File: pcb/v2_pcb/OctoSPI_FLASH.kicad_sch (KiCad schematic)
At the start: 7 parts, among them U5 MX25U51279GXDR00

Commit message: small
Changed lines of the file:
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@@
-	(wire
-		(pts
-			(xy 127 76.2) (xy 123.19 76.2)
-		)
-		(stroke
-			(width 0)
-			(type default)
-		)
-	)
 	(wire
 		(pts
@@
 	(wire
 		(pts
-			(xy 123.19 76.2) (xy 69.85 76.2)
+			(xy 69.85 76.2) (xy 127 76.2)
 		)
 		(stroke
@@
 		)
 	)
-	(embedded_fonts no)
 )

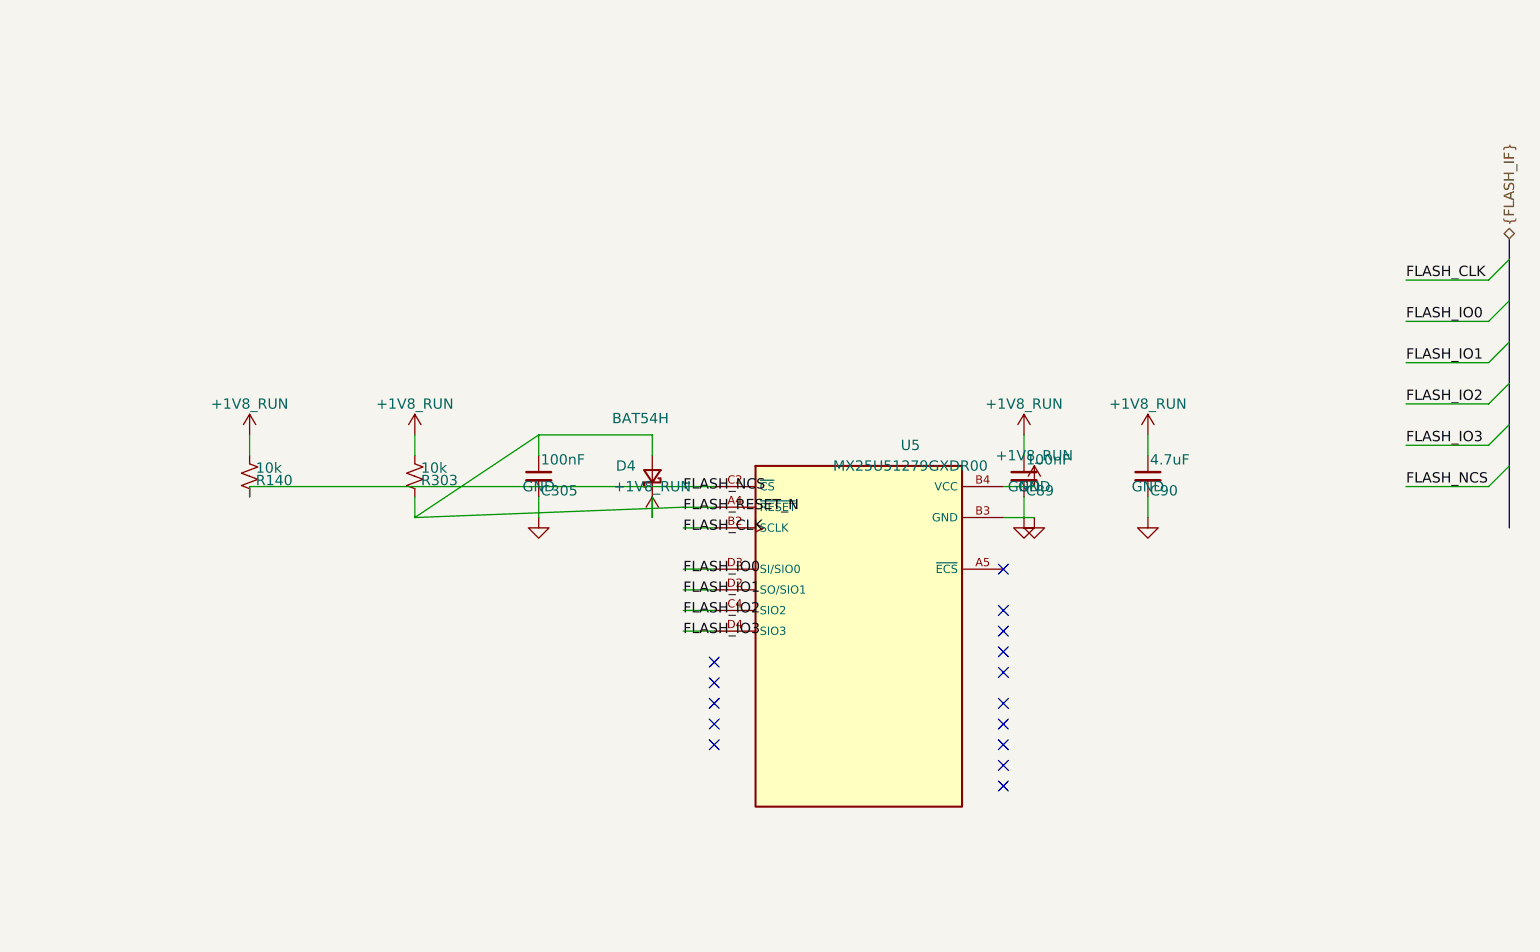
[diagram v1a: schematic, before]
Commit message: minor fixes
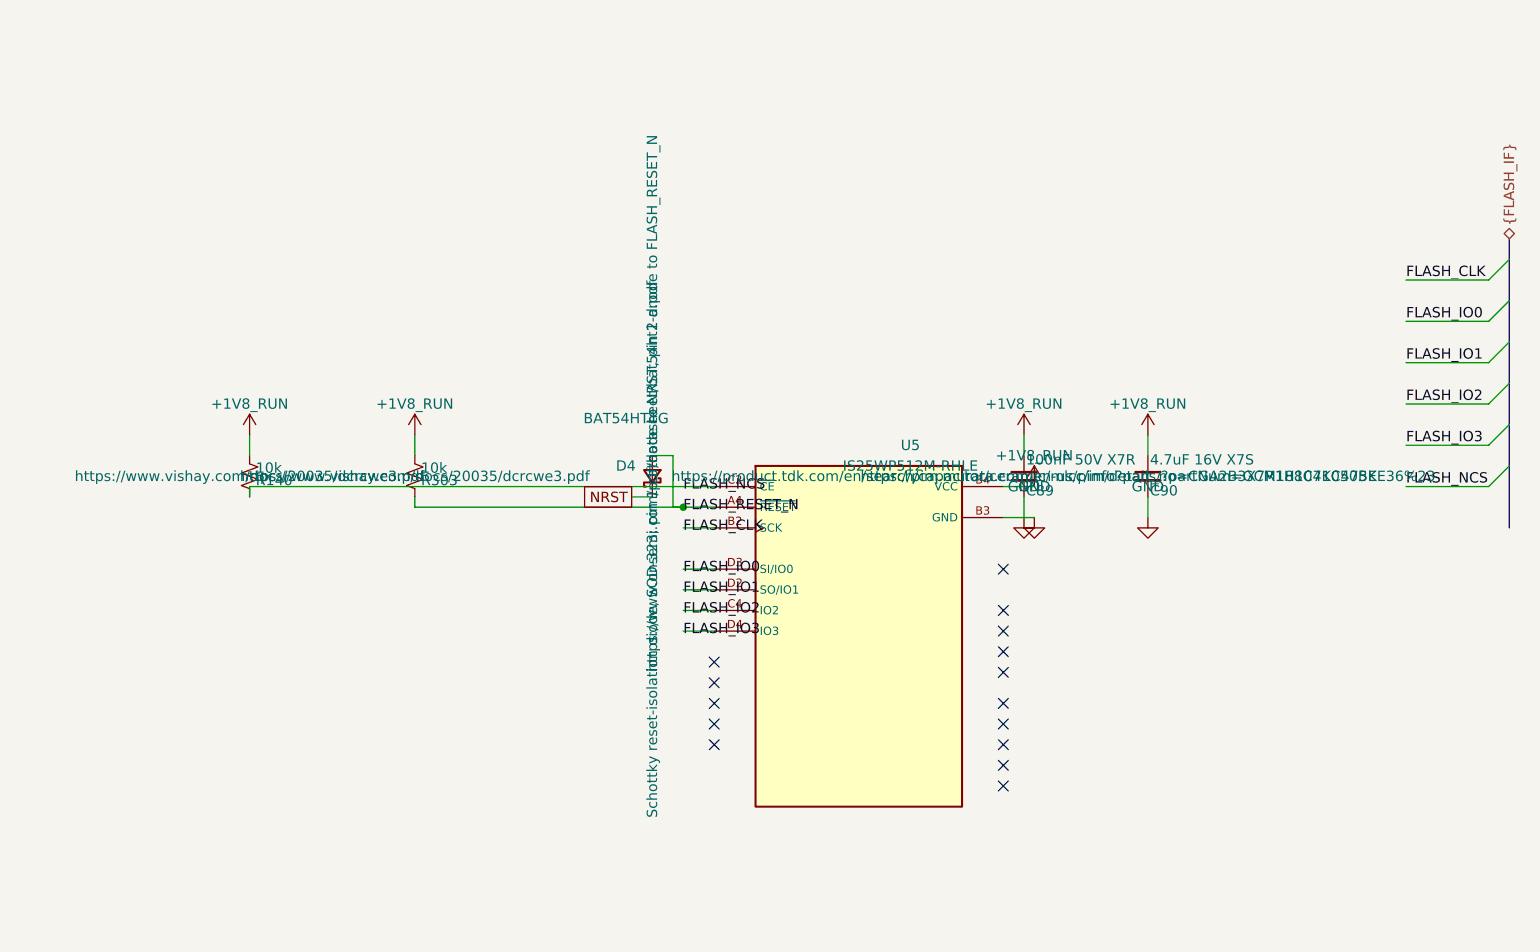
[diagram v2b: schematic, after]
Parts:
- removed C305: 100nF, Capacitor_SMD:C_0402_1005Metric, symbol Device:C_Small
- C89: value 100nF -> 100nF 50V X7R; Dielectric (none) -> X7R; MPN (none) -> CGA2B3X7R1H104K050BE; Manufacturer (none) -> TDK; Qualification (none) -> AEC-Q200; Termination (none) -> Soft termination; Tolerance (none) -> ±10%; Voltage (none) -> 50 VDC
- C90: value 4.7uF -> 4.7uF 16V X7S; Dielectric (none) -> X7S; MPN (none) -> GCM188C71C475KE36D; Manufacturer (none) -> Murata; Qualification (none) -> AEC-Q200 powertrain/safety; Tolerance (none) -> ±10%; Voltage (none) -> 16 VDC
- D4: value BAT54H -> BAT54HT1G; MPN BAT54H,115 -> BAT54HT1G; Manufacturer Nexperia -> onsemi
- R140: MPN (none) -> CRCW040210K0FKED; Manufacturer (none) -> Vishay; Power (none) -> 0.063 W; TCR (none) -> ±100 ppm/K; Tolerance (none) -> ±1%
- R303: MPN (none) -> CRCW040210K0FKED; Manufacturer (none) -> Vishay; Power (none) -> 0.063 W; Qualification (none) -> AEC-Q200; TCR (none) -> ±100 ppm/K; Tolerance (none) -> ±1%
- U5: value MX25U51279GXDR00 -> IS25WP512M-RHLE; symbol MX25U51279GXDR00:MX25U51279GXDR00 -> open-race-v2:IS25WP512M-RHLE; MPN MX25U51279GXDR00 -> IS25WP512M-RHLE; Manufacturer Macronix -> ISSI
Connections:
- net +1V8_RUN: no longer D4.1 (K)
- new net NRST: D4.1 (K)

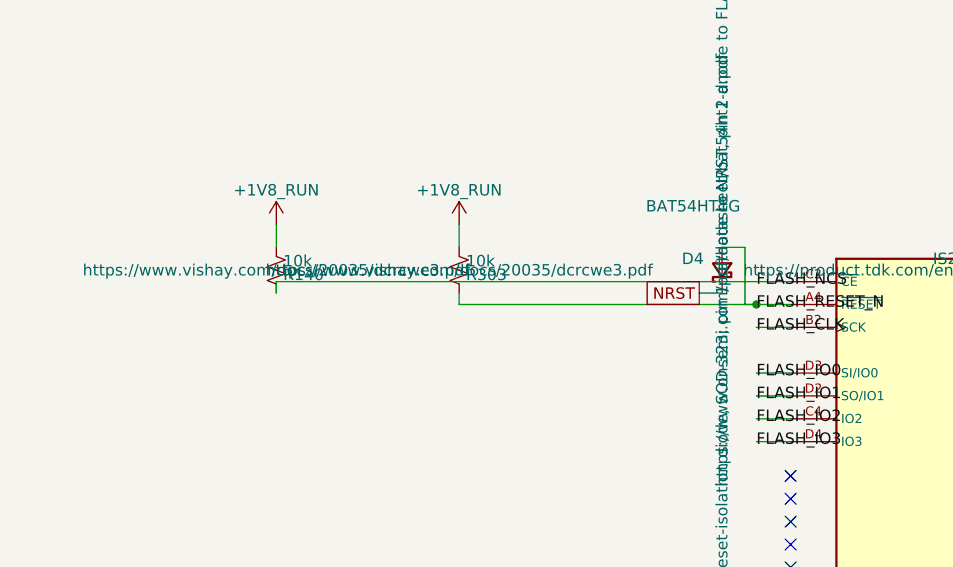
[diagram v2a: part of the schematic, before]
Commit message: pcb
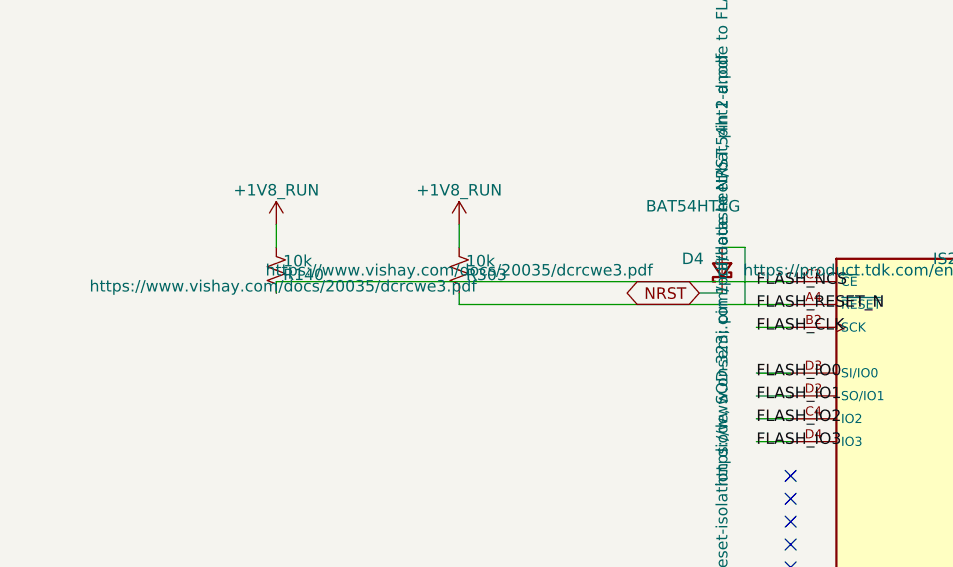
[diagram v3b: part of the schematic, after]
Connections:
- net FLASH_RESET_N: no longer D4.2 (A)

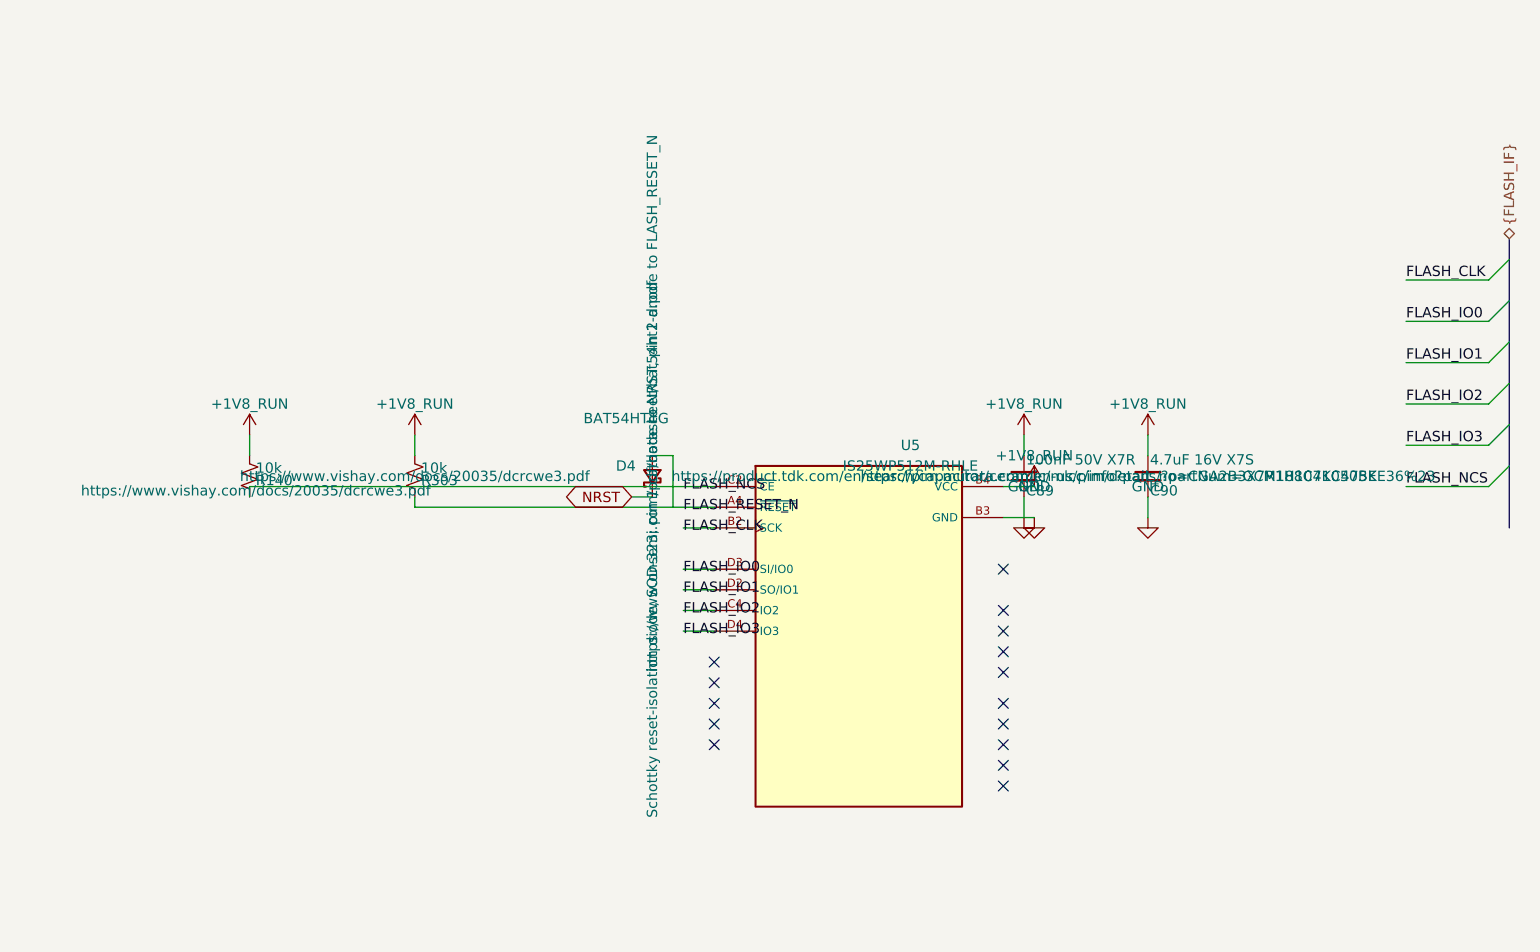
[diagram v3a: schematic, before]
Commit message: pcb flash
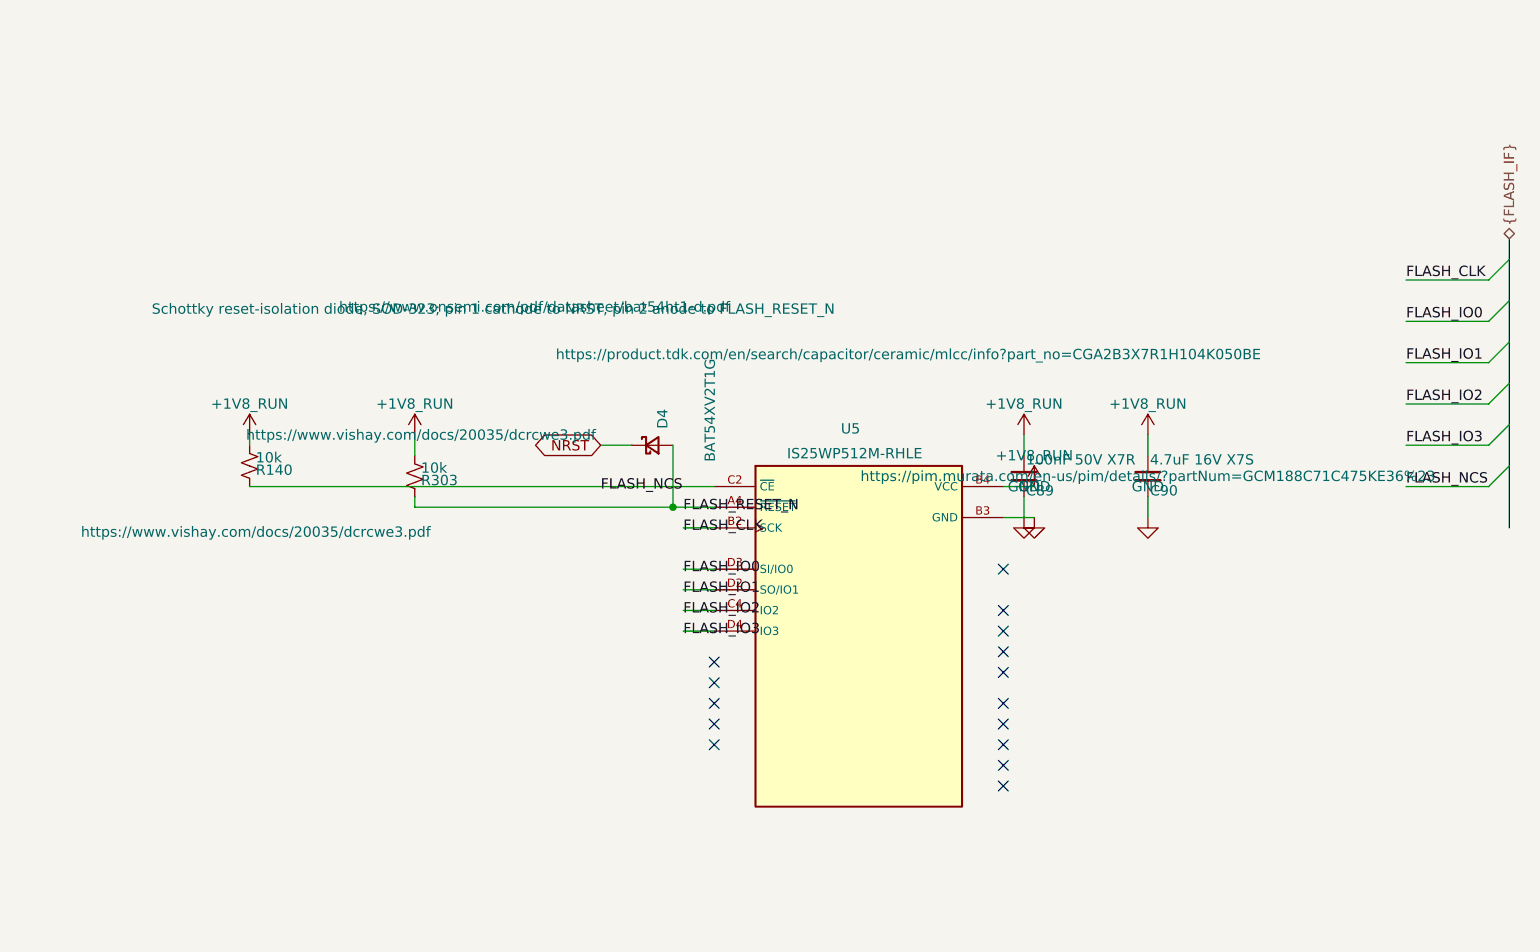
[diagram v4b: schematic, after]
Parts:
- D4: value BAT54HT1G -> BAT54XV2T1G; footprint Diode_SMD:D_SOD-323 -> Diode_SMD:D_SOD-523
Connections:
- net FLASH_RESET_N: now also D4.2 (A)
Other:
- moved on the sheet: D4, R140
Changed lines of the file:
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@@
 	(generator_version "10.0")
 	(paper "A4")
+	(junction
+		(at 121.92 78.74)
+		(diameter 0)
+		(color 0 0 0 0)
+	)
 	(no_connect
 		(at 162.56 107.95)
@@
 	(wire
 		(pts
-			(xy 121.92 72.39) (xy 121.92 78.74)
-		)
-		(stroke
-			(width 0)
-			(type default)
-		)
-	)
-	(wire
-		(pts
 			(xy 127 93.98) (xy 123.19 93.98)
 		)
@@
 	(wire
 		(pts
+			(xy 121.92 71.12) (xy 121.92 78.74)
+		)
+		(stroke
+			(width 0)
+			(type default)
+		)
+	)
+	(wire
+		(pts
 			(xy 180.34 72.39) (xy 180.34 69.85)
 		)
@@
 	(wire
 		(pts
-			(xy 119.38 77.47) (xy 116.84 77.47)
+			(xy 113.03 71.12) (xy 116.84 71.12)
 		)
 		(stroke
@@
 	(wire
 		(pts
-			(xy 69.85 72.39) (xy 69.85 69.85)
+			(xy 69.85 71.12) (xy 69.85 69.85)
 		)
 		(stroke
@@
 	(wire
 		(pts
-			(xy 69.85 76.2) (xy 69.85 77.47)
-		)
-		(stroke
-			(width 0)
-			(type default)
-		)
-	)
-	(wire
-		(pts
-			(xy 119.38 72.39) (xy 121.92 72.39)
-		)
-		(stroke
-			(width 0)
-			(type default)
-		)
-	)
-	(wire
-		(pts
-			(xy 90.17 78.74) (xy 127 78.74)
+			(xy 121.92 78.74) (xy 127 78.74)
+		)
+		(stroke
+			(width 0)
+			(type default)
+		)
+	)
+	(wire
+		(pts
+			(xy 90.17 78.74) (xy 121.92 78.74)
 		)
 		(stroke
@@
 	)
 	(label "FLASH_NCS"
-		(at 123.19 76.2 0)
+		(at 113.03 76.2 0)
 		(effects
 			(font
@@
 	(global_label "NRST"
 		(shape bidirectional)
-		(at 116.84 77.47 180)
+		(at 113.03 71.12 180)
 		(effects
 			(font
@@
 		)
 		(property "Intersheetrefs" "${INTERSHEET_REFS}"
-			(at 116.84 77.47 0)
+			(at 113.03 71.12 0)
 			(hide yes)
 			(show_name no)
@@
 		(in_pos_files yes)
 		(dnp no)
-		(fields_autoplaced yes)
 		(property "Reference" "U5"
-			(at 151.13 71.12 0)
+			(at 143.764 69.088 0)
 			(show_name no)
 			(do_not_autoplace no)
@@
 		)
 		(property "Value" "IS25WP512M-RHLE"
-			(at 151.13 73.66 0)
+			(at 144.272 72.136 0)
 			(show_name no)
 			(do_not_autoplace no)
@@
 		)
 		(property "Datasheet" "https://product.tdk.com/en/search/capacitor/ceramic/mlcc/info?part_no=CGA2B3X7R1H104K050BE"
-			(at 165.1 74.93 0)
+			(at 150.876 59.944 0)
 			(show_name no)
 			(do_not_autoplace no)
@@
 		)
 		(property "Datasheet" "https://www.vishay.com/docs/20035/dcrcwe3.pdf"
-			(at 90.17 74.93 0)
+			(at 90.932 69.85 0)
 			(show_name no)
 			(do_not_autoplace no)
@@
 	(symbol
 		(lib_id "Device:R_Small_US")
-		(at 69.85 74.93 0)
+		(at 69.85 73.66 0)
 		(unit 1)
 		(body_style 1)
@@
 		(dnp no)
 		(property "Reference" "R140"
-			(at 70.612 75.438 0)
+			(at 70.612 74.168 0)
 			(show_name no)
 			(do_not_autoplace no)
@@
 		)
 		(property "Value" "10k"
-			(at 70.612 73.914 0)
+			(at 70.612 72.644 0)
 			(show_name no)
 			(do_not_autoplace no)
@@
 		)
 		(property "Footprint" "Resistor_SMD:R_0402_1005Metric"
-			(at 69.85 74.93 0)
+			(at 69.85 73.66 0)
 			(hide yes)
 			(show_name no)
@@
 		)
 		(property "Datasheet" "https://www.vishay.com/docs/20035/dcrcwe3.pdf"
-			(at 70.612 76.708 0)
+			(at 70.612 81.788 0)
 			(show_name no)
 			(do_not_autoplace no)
@@
 		)
 		(property "Description" ""
-			(at 69.85 74.93 0)
+			(at 69.85 73.66 0)
 			(show_name no)
 			(do_not_autoplace no)
@@
 		)
 		(property "Manufacturer" "Vishay"
-			(at 69.85 74.93 0)
+			(at 69.85 73.66 0)
 			(hide yes)
 			(show_name no)
@@
 		)
 		(property "MPN" "CRCW040210K0FKED"
-			(at 69.85 74.93 0)
+			(at 69.85 73.66 0)
 			(hide yes)
 			(show_name no)
@@
 		)
 		(property "Tolerance" "±1%"
-			(at 69.85 74.93 0)
+			(at 69.85 73.66 0)
 			(hide yes)
 			(show_name no)
@@
 		)
 		(property "Power" "0.063 W"
-			(at 69.85 74.93 0)
+			(at 69.85 73.66 0)
 			(hide yes)
 			(show_name no)
@@
 		)
 		(property "TCR" "±100 ppm/K"
-			(at 69.85 74.93 0)
+			(at 69.85 73.66 0)
 			(hide yes)
 			(show_name no)
@@
 	(symbol
 		(lib_id "Device:D_Schottky_Small")
-		(at 119.38 74.93 90)
+		(at 119.38 71.12 0)
 		(unit 1)
 		(body_style 1)
@@
 		(dnp no)
 		(property "Reference" "D4"
-			(at 117.348 73.66 90)
+			(at 120.65 69.088 90)
 			(show_name no)
 			(do_not_autoplace no)
@@
 			)
 		)
-		(property "Value" "BAT54HT1G"
-			(at 121.412 67.818 90)
+		(property "Value" "BAT54XV2T1G"
+			(at 126.492 73.152 90)
 			(show_name no)
 			(do_not_autoplace no)
@@
 			)
 		)
-		(property "Footprint" "Diode_SMD:D_SOD-323"
-			(at 119.38 74.93 90)
+		(property "Footprint" "Diode_SMD:D_SOD-523"
+			(at 119.38 71.12 90)
 			(hide yes)
 			(show_name no)
@@
 		)
 		(property "Datasheet" "https://www.onsemi.com/pdf/datasheet/bat54ht1-d.pdf"
-			(at 119.38 74.93 0)
+			(at 104.902 54.102 0)
 			(show_name no)
 			(do_not_autoplace no)
@@
 		)
 		(property "Description" "Schottky reset-isolation diode, SOD-323; pin 1 cathode to NRST, pin 2 anode to FLASH_RESET_N"
-			(at 119.38 74.93 0)
+			(at 99.822 54.356 0)
 			(show_name no)
 			(do_not_autoplace no)
@@
 		)
 		(property "MPN" "BAT54HT1G"
-			(at 121.92 80.0099 0)
+			(at 114.3001 73.66 0)
 			(hide yes)
 			(show_name no)
@@
 		)
 		(property "Manufacturer" "onsemi"
-			(at 121.92 80.0099 0)
-			(hide yes)
-			(show_name no)
+			(at 114.3001 73.66 0)
+			(hide yes)
+			(show_name no)
